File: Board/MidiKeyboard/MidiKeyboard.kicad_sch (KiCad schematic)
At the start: 33 parts, among them J1 USB_C_Receptacle_USB2.0_16P, J2 Bat, J3 Boot, Q1 DMP3099L, SW1 CK_KMS2xxG, U1 ESP32-C3, U2 XC6220B331MR, U3 TP4056-42-ESOP8, U4 TCA8418RTWR

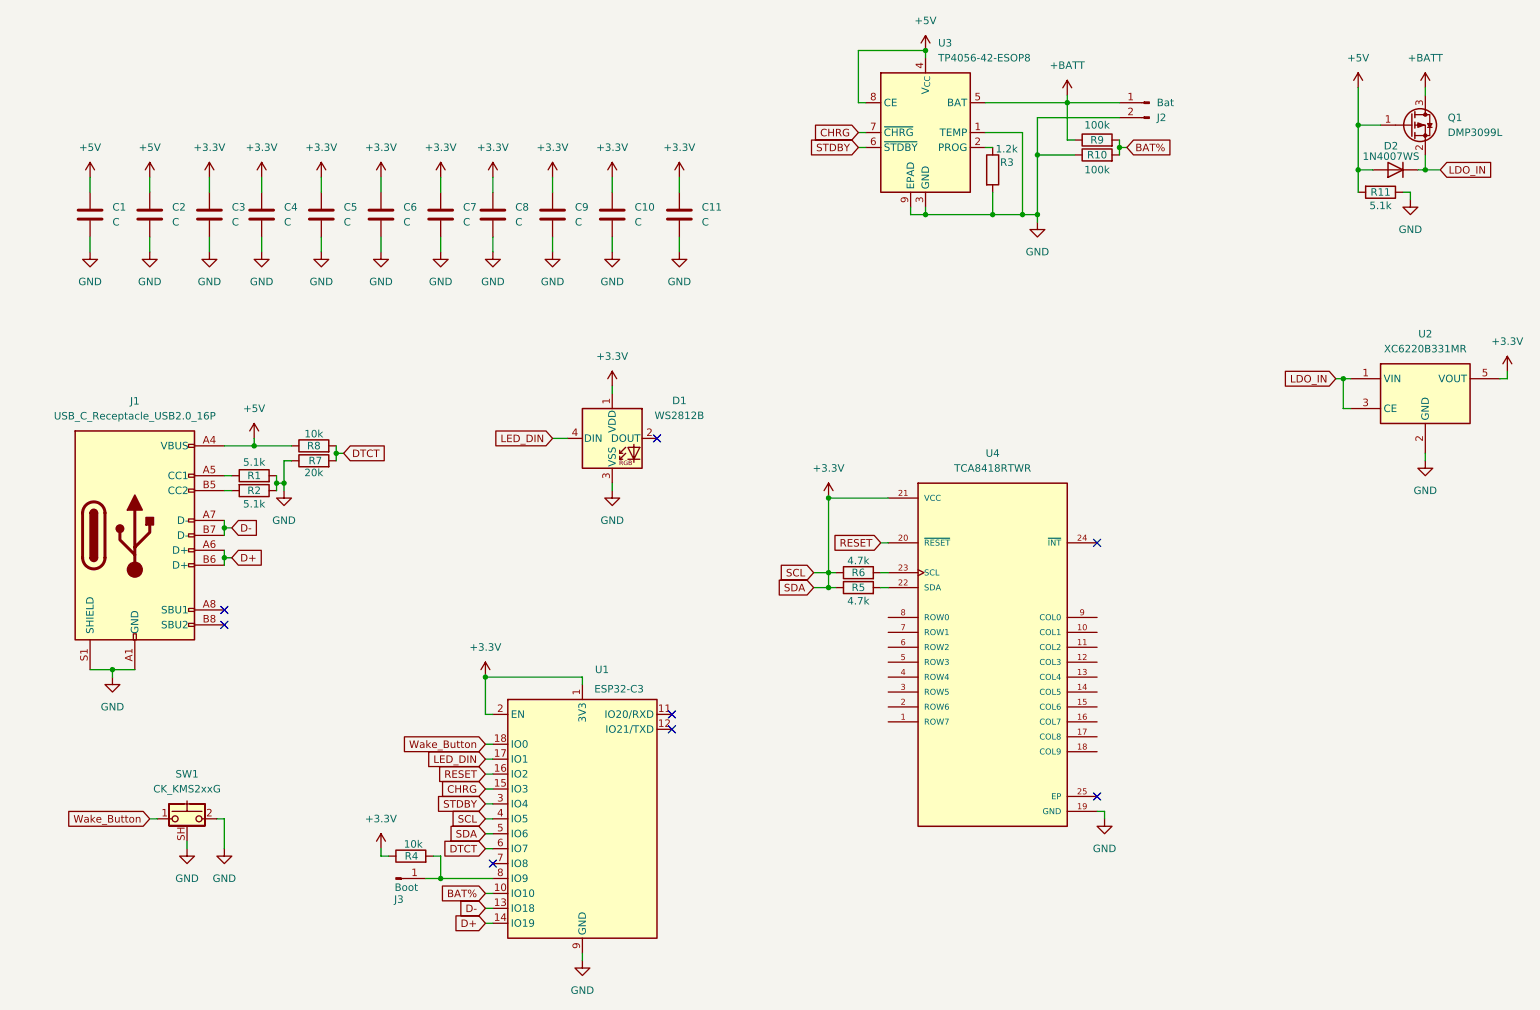
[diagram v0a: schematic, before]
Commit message: Complete Schema + Starting PCB
Anythink may be changed
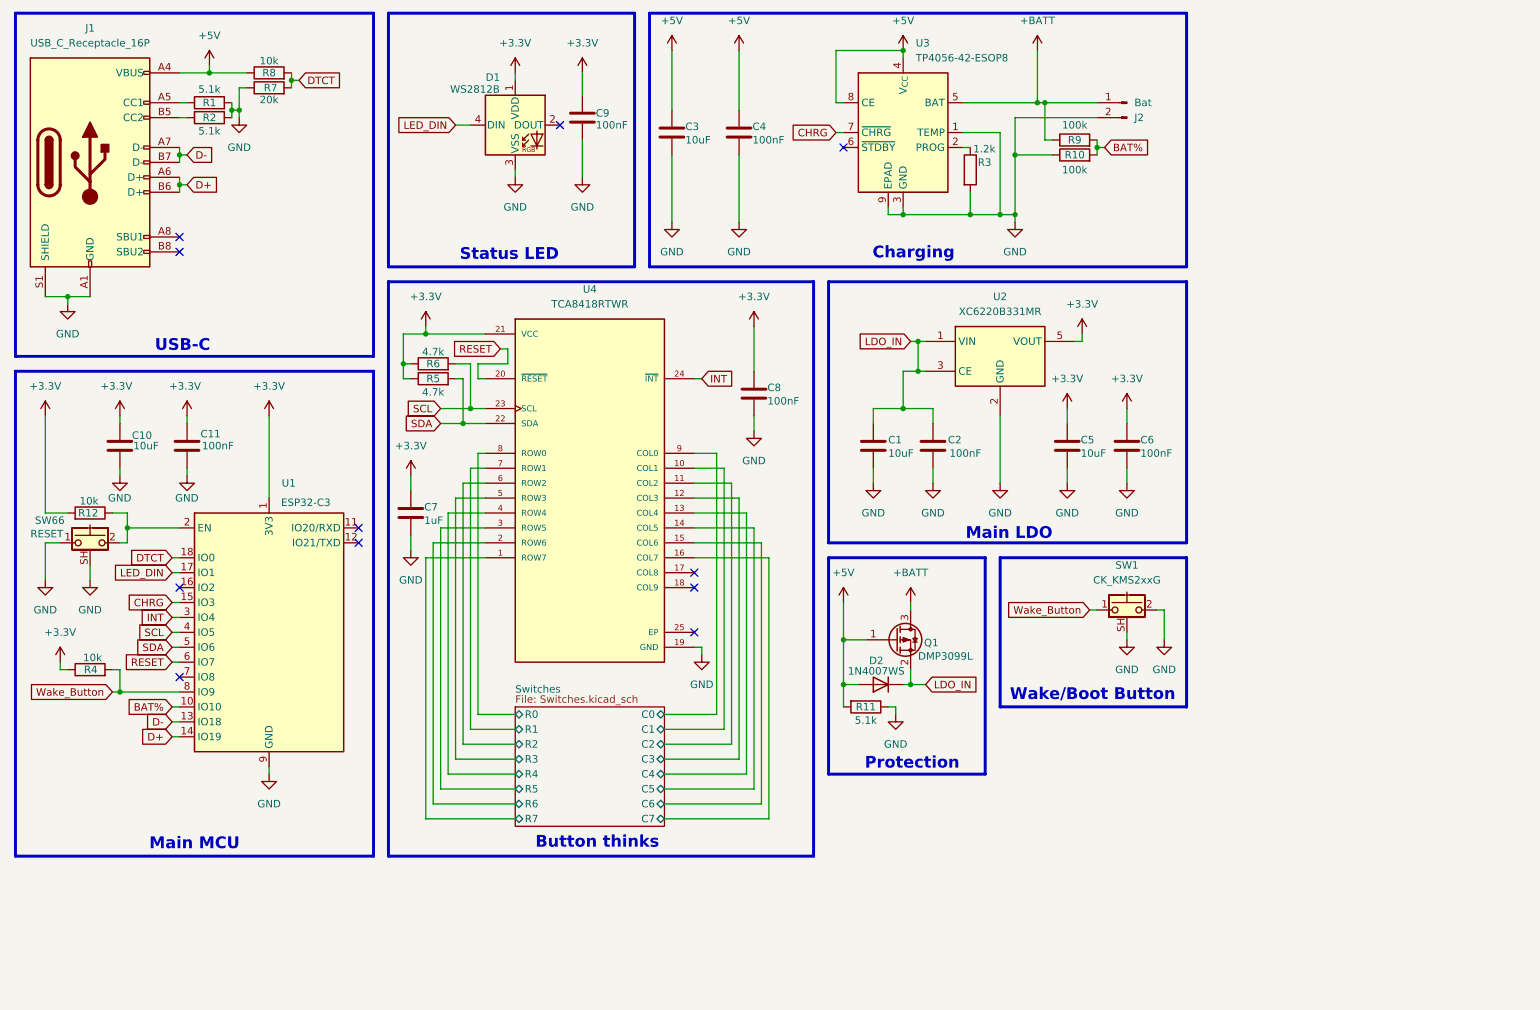
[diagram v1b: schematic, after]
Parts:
- removed J3: Boot, symbol Connector:Conn_01x01_Pin
- added R12: 10k, Resistor_SMD:R_0402_1005Metric, symbol Device:R
- added SW66: RESET, Button_Switch_SMD:SW_SPST_CK_KMS2xxGP, symbol Switch:CK_KMS2xxG
- C1, C10, C3, C5: value C -> 10uF; footprint (none) -> Capacitor_SMD:C_0402_1005Metric
- C11, C2, C4, C6, C8, C9: value C -> 100nF; footprint (none) -> Capacitor_SMD:C_0402_1005Metric
- C7: value C -> 1uF; footprint (none) -> Capacitor_SMD:C_0402_1005Metric
- D2: footprint (none) -> Diode_SMD:D_0402_1005Metric
- J1: value USB_C_Receptacle_USB2.0_16P -> USB_C_Receptacle_16P; footprint (none) -> Connector_USB:USB_C_Receptacle_HCTL_HC-TYPE-C-16P-01A
- J2: footprint (none) -> Connector_JST:JST_PH_B2B-PH-SM4-TB_1x02-1MP_P2.00mm_Vertical
- R1, R10, R11, R2, R3, R4, R5, R6, R7, R8, R9: footprint (none) -> Resistor_SMD:R_0402_1005Metric
- U4: footprint (none) -> MidiKey:QFN50P400X400X80-25N
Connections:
- net +3.3V: now also R12.2; no longer C3.1, C4.1, U1.2 (EN), U1.4 (IO5), U1.5 (IO6)
- net +5V: now also C3.1, C4.1; no longer C1.1, C2.1
- net DTCT: now also U1.18 (IO0); no longer U1.6 (IO7)
- net GND: now also SW66.1, SW66.SH (B)
- net LDO_IN: now also C1.1, C2.1
- net RESET: now also U1.6 (IO7); no longer U1.16 (IO2)
- net Wake_Button: now also R4.2, U1.8 (IO9); no longer U1.18 (IO0)
- net SDA: now reaches R5.2, U4.22 (SDA)
- net SDA: now also U1.5 (IO6)
- net Switches/R7: now reaches U4.1 (ROW7)
- net Switches/C1: now reaches U4.10 (COL1)
- net Switches/C2: now reaches U4.11 (COL2)
- net Switches/C3: now reaches U4.12 (COL3)
- net Switches/C4: now reaches U4.13 (COL4)
- net Switches/C5: now reaches U4.14 (COL5)
- net Switches/C6: now reaches U4.15 (COL6)
- net Switches/C7: now reaches U4.16 (COL7)
- net Switches/R6: now reaches U4.2 (ROW6)
- net SCL: now reaches R6.2, U4.23 (SCL)
- net SCL: now also U1.4 (IO5)
- net INT: now reaches U4.24 (~{INT})
- net INT: now also U1.3 (IO4)
- net Switches/R5: now reaches U4.3 (ROW5)
- net Switches/R4: now reaches U4.4 (ROW4)
- net Switches/R3: now reaches U4.5 (ROW3)
- net Switches/R2: now reaches U4.6 (ROW2)
- net Switches/R1: now reaches U4.7 (ROW1)
- net Switches/R0: now reaches U4.8 (ROW0)
- net Switches/C0: now reaches U4.9 (COL0)
- net STDBY: no longer names the net of U3.6 (~{STDBY})
- net STDBY: no longer U1.3 (IO4)
- new net: R12.1, SW66.2, U1.2 (EN)
- no-connect marks 8 -> 11
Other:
- added sheet Switches (Switches.kicad_sch)
- note added: "Button thinks"
- note added: "Charging"
- note added: "Main LDO"
- note added: "Main MCU"
- note added: "Protection"
- note added: "Status LED"
- note added: "USB-C"
- note added: "Wake/Boot Button"
- moved on the sheet: C1, C10, C11, C2, C3, C4, C5, C6, C7, C8, C9, D1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
